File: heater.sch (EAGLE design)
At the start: 9 parts, among them Q1 irfz44n, Q2 2N2907, T1 2N2222

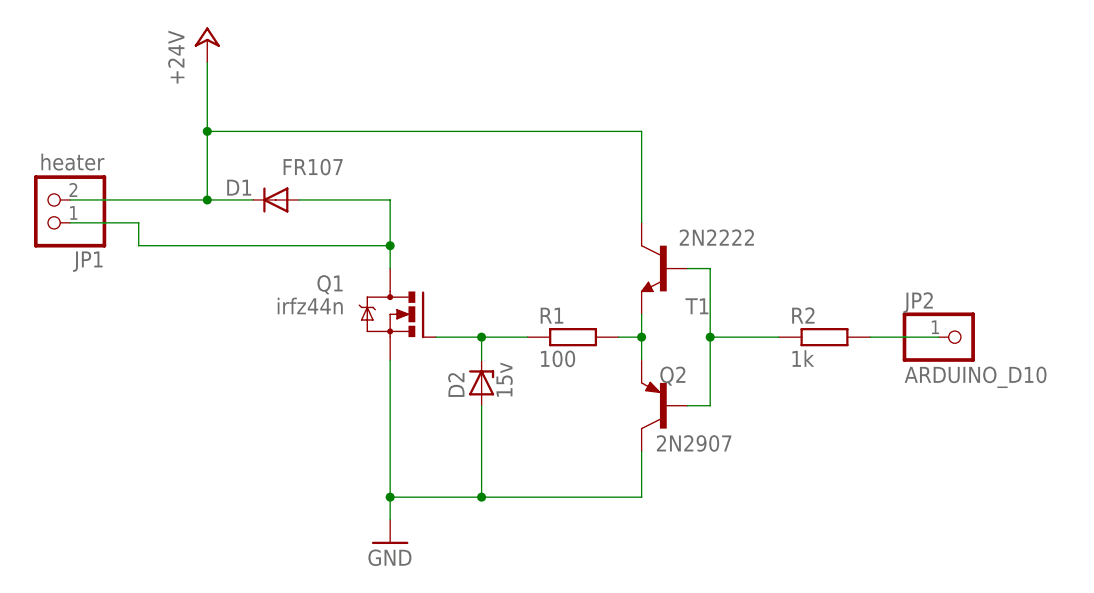
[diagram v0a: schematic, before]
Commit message: Add files via upload
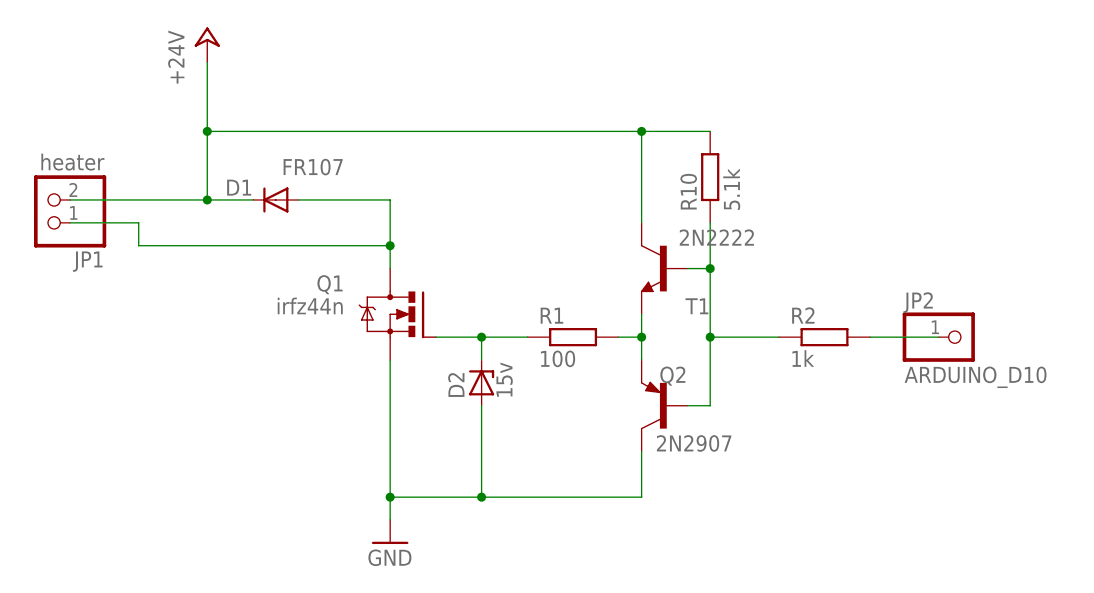
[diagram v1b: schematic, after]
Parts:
- added R10: 5.1k, rcl:R-EU_0204/5
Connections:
- net +24V: now also R10.2
- net N$5: now also R10.1
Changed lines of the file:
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@@
 <part name="P+1" library="supply1" library_urn="urn:adsk.eagle:library:371" deviceset="+24V" device=""/>
 <part name="JP2" library="pinhead" library_urn="urn:adsk.eagle:library:325" deviceset="PINHD-1X1" device="" package3d_urn="urn:adsk.eagle:package:22485/2" value="ARDUINO_D10"/>
+<part name="R10" library="rcl" library_urn="urn:adsk.eagle:library:334" deviceset="R-EU_" device="0204/5" package3d_urn="urn:adsk.eagle:package:23488/1" value="5.1k"/>
 </parts>
 <sheets>
@@
 <attribute name="VALUE" x="80.01" y="58.42" size="1.778" layer="96"/>
 </instance>
+<instance part="R10" gate="G$1" x="58.42" y="81.28" rot="R90">
+<attribute name="NAME" x="56.9214" y="77.47" size="1.778" layer="95" rot="R90"/>
+<attribute name="VALUE" x="61.722" y="77.47" size="1.778" layer="96" rot="R90"/>
+</instance>
 </instances>
 <busses>
@@
 <wire x1="50.8" y1="86.36" x2="2.54" y2="86.36" width="0.1524" layer="91"/>
 <junction x="2.54" y="86.36"/>
+<pinref part="R10" gate="G$1" pin="2"/>
+<wire x1="58.42" y1="86.36" x2="50.8" y2="86.36" width="0.1524" layer="91"/>
+<junction x="50.8" y="86.36"/>
 </segment>
 </net>
@@
 <wire x1="66.04" y1="63.5" x2="58.42" y2="63.5" width="0.1524" layer="91"/>
 <junction x="58.42" y="63.5"/>
+<pinref part="R10" gate="G$1" pin="1"/>
+<wire x1="58.42" y1="76.2" x2="58.42" y2="71.12" width="0.1524" layer="91"/>
+<junction x="58.42" y="71.12"/>
 </segment>
 </net>

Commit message: Add files via upload
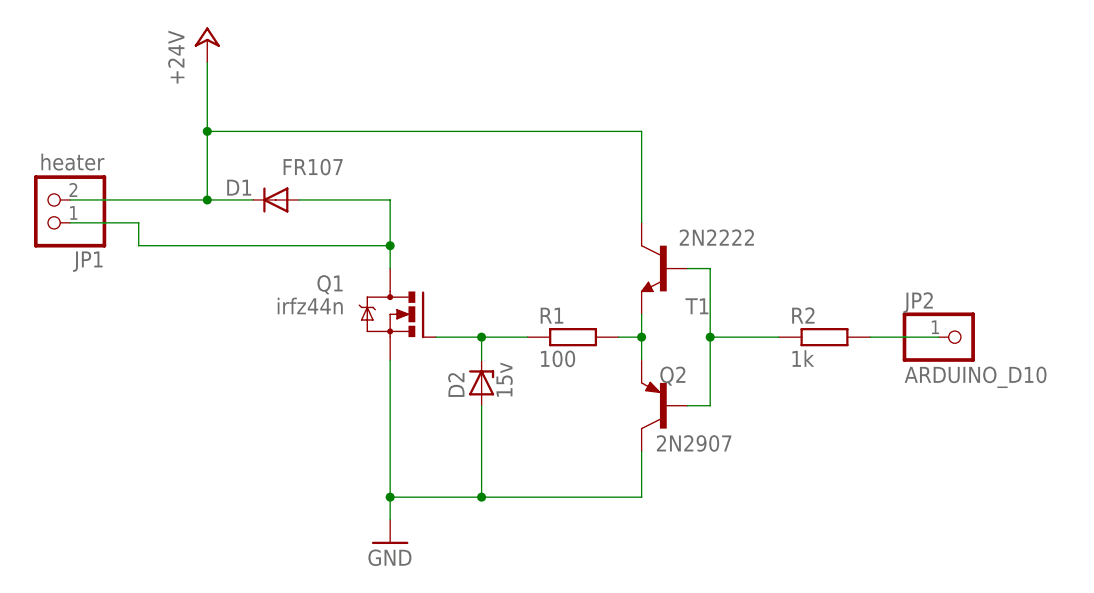
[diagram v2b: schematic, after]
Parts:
- removed R10: 5.1k, rcl:R-EU_0204/5
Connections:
- net +24V: no longer R10.2
- net N$5: no longer R10.1
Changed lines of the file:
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@@
 <part name="P+1" library="supply1" library_urn="urn:adsk.eagle:library:371" deviceset="+24V" device=""/>
 <part name="JP2" library="pinhead" library_urn="urn:adsk.eagle:library:325" deviceset="PINHD-1X1" device="" package3d_urn="urn:adsk.eagle:package:22485/2" value="ARDUINO_D10"/>
-<part name="R10" library="rcl" library_urn="urn:adsk.eagle:library:334" deviceset="R-EU_" device="0204/5" package3d_urn="urn:adsk.eagle:package:23488/1" value="5.1k"/>
 </parts>
 <sheets>
@@
 <attribute name="VALUE" x="80.01" y="58.42" size="1.778" layer="96"/>
 </instance>
-<instance part="R10" gate="G$1" x="58.42" y="81.28" rot="R90">
-<attribute name="NAME" x="56.9214" y="77.47" size="1.778" layer="95" rot="R90"/>
-<attribute name="VALUE" x="61.722" y="77.47" size="1.778" layer="96" rot="R90"/>
-</instance>
 </instances>
 <busses>
@@
 <wire x1="50.8" y1="86.36" x2="2.54" y2="86.36" width="0.1524" layer="91"/>
 <junction x="2.54" y="86.36"/>
-<pinref part="R10" gate="G$1" pin="2"/>
-<wire x1="58.42" y1="86.36" x2="50.8" y2="86.36" width="0.1524" layer="91"/>
-<junction x="50.8" y="86.36"/>
 </segment>
 </net>
@@
 <wire x1="66.04" y1="63.5" x2="58.42" y2="63.5" width="0.1524" layer="91"/>
 <junction x="58.42" y="63.5"/>
-<pinref part="R10" gate="G$1" pin="1"/>
-<wire x1="58.42" y1="76.2" x2="58.42" y2="71.12" width="0.1524" layer="91"/>
-<junction x="58.42" y="71.12"/>
 </segment>
 </net>
